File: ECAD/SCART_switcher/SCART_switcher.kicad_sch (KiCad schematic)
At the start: 8 parts

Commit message: Progressed ECAD.
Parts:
- H1, H2, H3, H4, H5, H6, H7, H8: MPN (none) -> N/A; Status (none) -> OK
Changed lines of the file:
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@@
+      (effects (font (size 1.27 1.27)) hide)
+    )
+    (property "Status" "OK" (at 195.58 158.75 0)
+      (effects (font (size 1.27 1.27)) hide)
+    )
+    (property "MPN" "N/A" (at 195.58 158.75 0)
       (effects (font (size 1.27 1.27)) hide)
     )
@@
       (effects (font (size 1.27 1.27)) hide)
     )
+    (property "Status" "OK" (at 195.58 152.4 0)
+      (effects (font (size 1.27 1.27)) hide)
+    )
+    (property "MPN" "N/A" (at 195.58 152.4 0)
+      (effects (font (size 1.27 1.27)) hide)
+    )
     (instances
       (project "SCART_switcher"
@@
       (effects (font (size 1.27 1.27)) hide)
     )
+    (property "Status" "OK" (at 236.22 152.4 0)
+      (effects (font (size 1.27 1.27)) hide)
+    )
+    (property "MPN" "N/A" (at 236.22 152.4 0)
+      (effects (font (size 1.27 1.27)) hide)
+    )
     (instances
       (project "SCART_switcher"
@@
       (effects (font (size 1.27 1.27)) hide)
     )
+    (property "Status" "OK" (at 236.22 158.75 0)
+      (effects (font (size 1.27 1.27)) hide)
+    )
+    (property "MPN" "N/A" (at 236.22 158.75 0)
+      (effects (font (size 1.27 1.27)) hide)
+    )
     (instances
       (project "SCART_switcher"
@@
       (effects (font (size 1.27 1.27)) hide)
     )
+    (property "Status" "OK" (at 215.9 158.75 0)
+      (effects (font (size 1.27 1.27)) hide)
+    )
+    (property "MPN" "N/A" (at 215.9 158.75 0)
+      (effects (font (size 1.27 1.27)) hide)
+    )
     (instances
       (project "SCART_switcher"
@@
       (effects (font (size 1.27 1.27)) hide)
     )
+    (property "Status" "OK" (at 256.54 152.4 0)
+      (effects (font (size 1.27 1.27)) hide)
+    )
+    (property "MPN" "N/A" (at 256.54 152.4 0)
+      (effects (font (size 1.27 1.27)) hide)
+    )
     (instances
       (project "SCART_switcher"
@@
       (effects (font (size 1.27 1.27)) hide)
     )
+    (property "Status" "OK" (at 256.54 158.75 0)
+      (effects (font (size 1.27 1.27)) hide)
+    )
+    (property "MPN" "N/A" (at 256.54 158.75 0)
+      (effects (font (size 1.27 1.27)) hide)
+    )
     (instances
       (project "SCART_switcher"
@@
       (effects (font (size 1.27 1.27)) hide)
     )
+    (property "Status" "OK" (at 215.9 152.4 0)
+      (effects (font (size 1.27 1.27)) hide)
+    )
+    (property "MPN" "N/A" (at 215.9 152.4 0)
+      (effects (font (size 1.27 1.27)) hide)
+    )

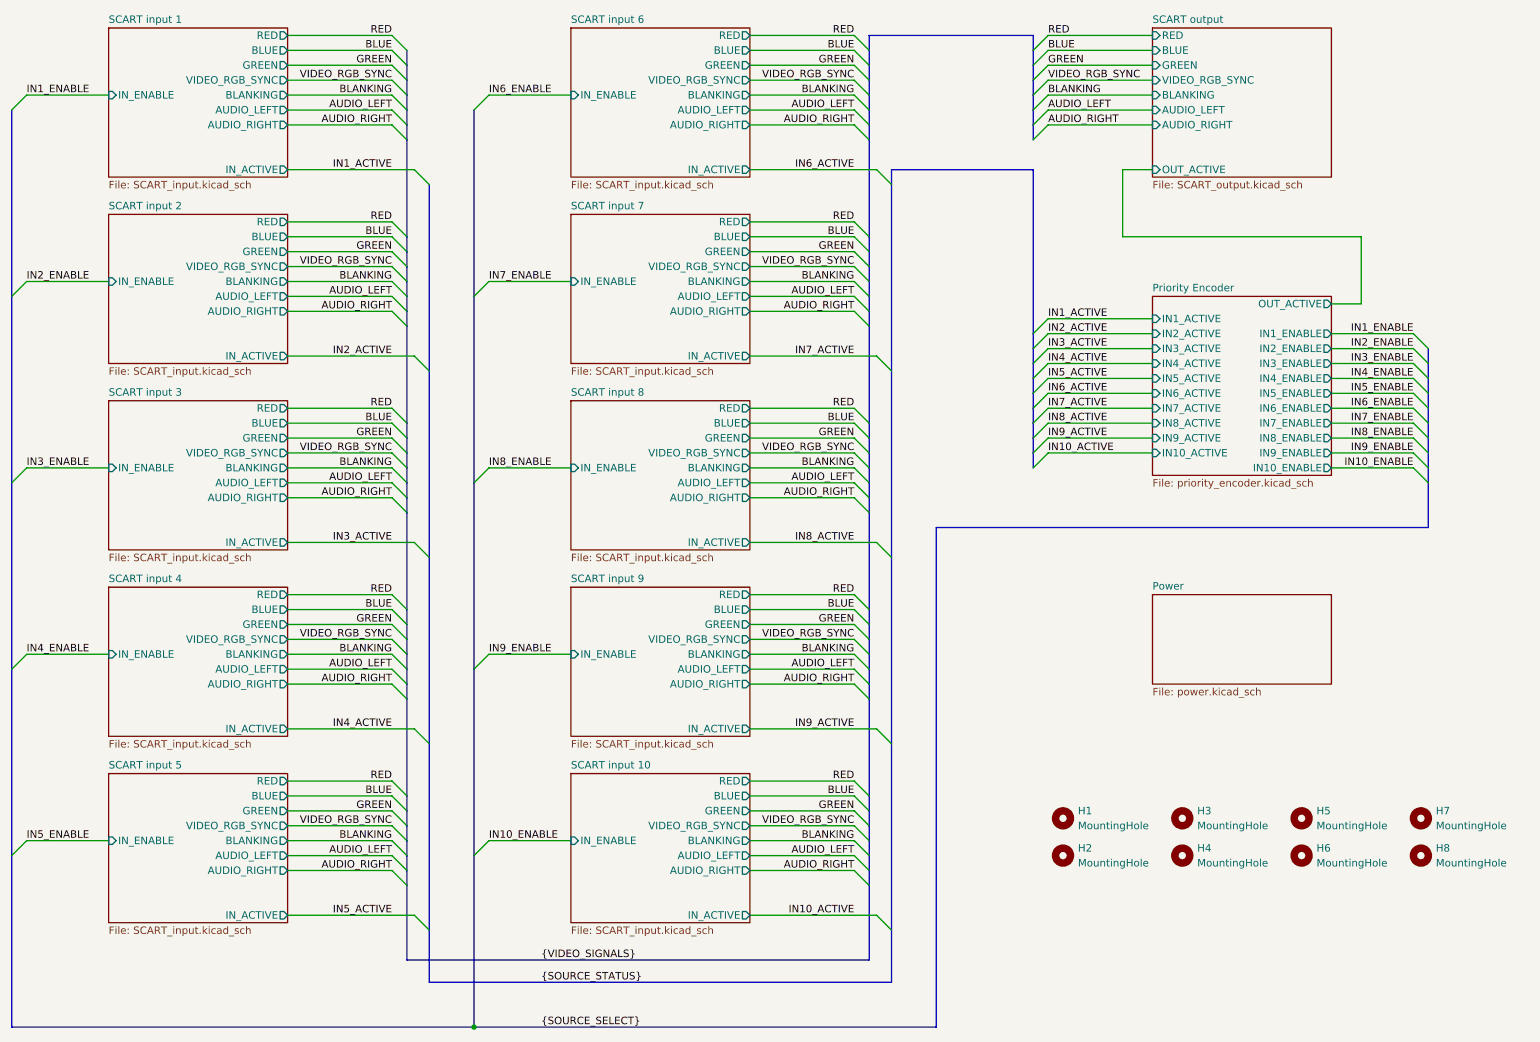
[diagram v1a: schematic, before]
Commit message: Progressed ECAD.
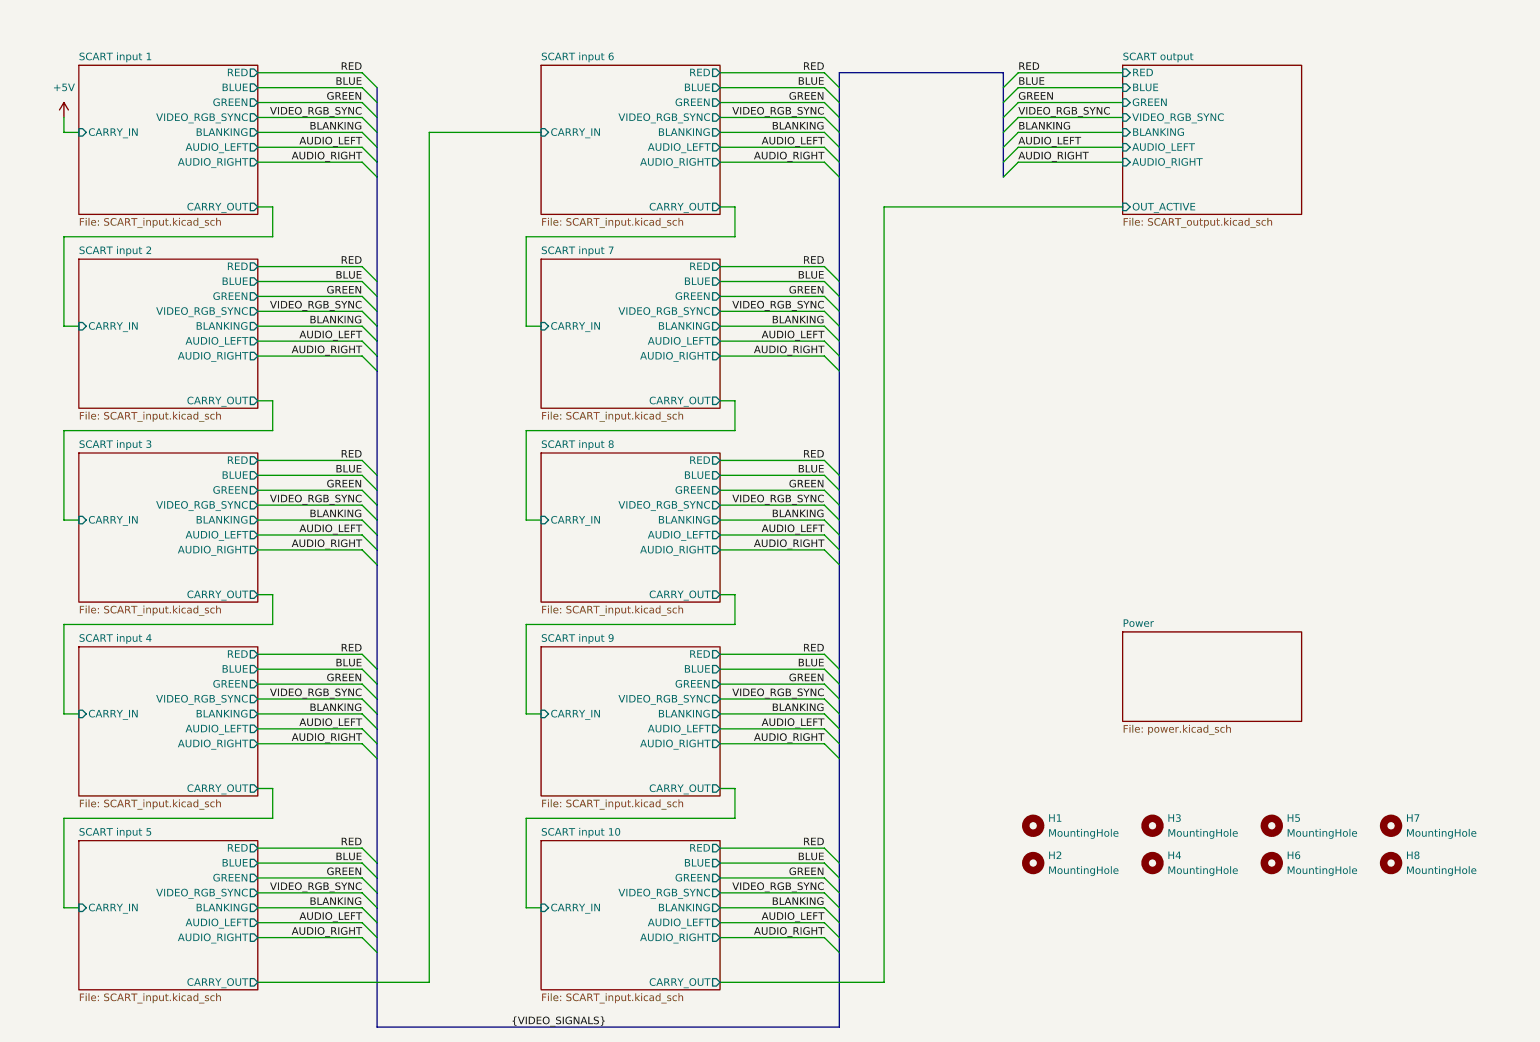
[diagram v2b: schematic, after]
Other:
- removed sheet Priority Encoder
- sheet SCART input 1 ports: added CARRY_IN, CARRY_OUT; removed IN_ACTIVE, IN_ENABLE
- sheet SCART input 10 ports: added CARRY_IN, CARRY_OUT; removed IN_ACTIVE, IN_ENABLE
- sheet SCART input 2 ports: added CARRY_IN, CARRY_OUT; removed IN_ACTIVE, IN_ENABLE
- sheet SCART input 3 ports: added CARRY_IN, CARRY_OUT; removed IN_ACTIVE, IN_ENABLE
- sheet SCART input 4 ports: added CARRY_IN, CARRY_OUT; removed IN_ACTIVE, IN_ENABLE
- sheet SCART input 5 ports: added CARRY_IN, CARRY_OUT; removed IN_ACTIVE, IN_ENABLE
- sheet SCART input 6 ports: added CARRY_IN, CARRY_OUT; removed IN_ACTIVE, IN_ENABLE
- sheet SCART input 7 ports: added CARRY_IN, CARRY_OUT; removed IN_ACTIVE, IN_ENABLE
- sheet SCART input 8 ports: added CARRY_IN, CARRY_OUT; removed IN_ACTIVE, IN_ENABLE
- sheet SCART input 9 ports: added CARRY_IN, CARRY_OUT; removed IN_ACTIVE, IN_ENABLE
- moved on the sheet: H1, H2, H3, H4, H5, H6, H7, H8
